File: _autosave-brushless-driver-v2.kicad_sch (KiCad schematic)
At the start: 22 parts, among them J1 Conn_01x07_Socket, J2 encoder_r, J5 encoder_l, U1 ESP32-WROOM-32E-R2

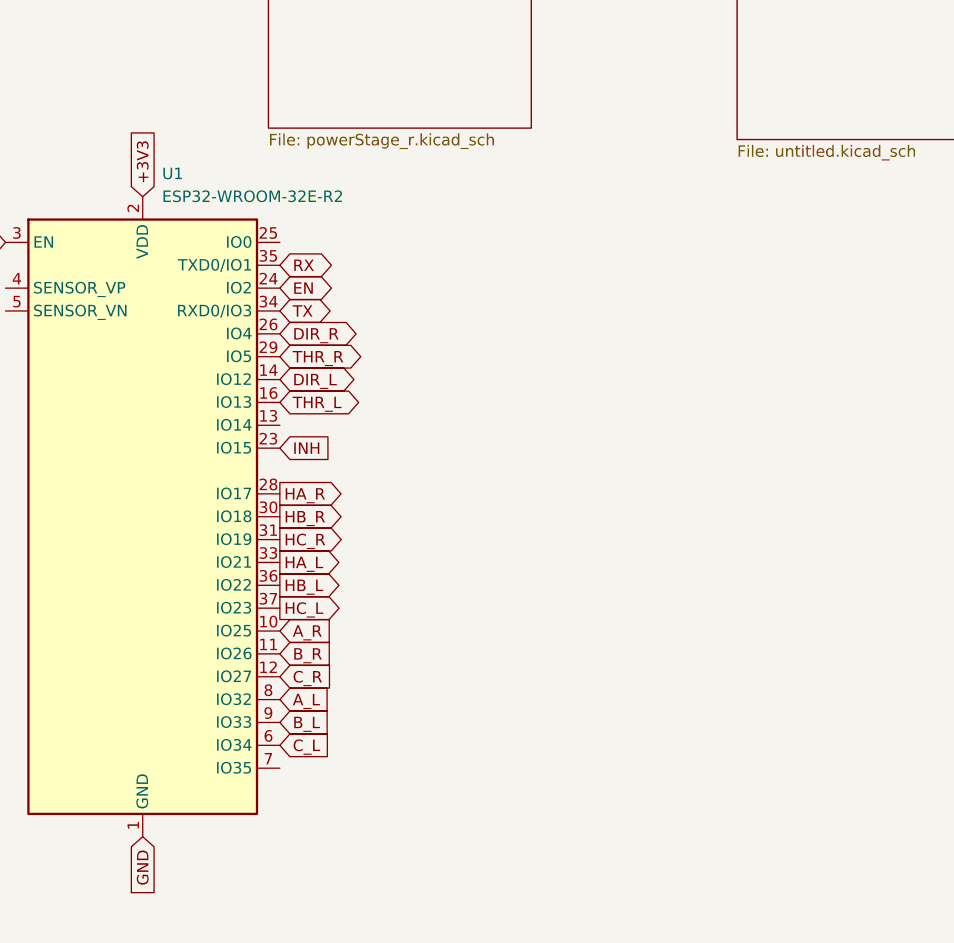
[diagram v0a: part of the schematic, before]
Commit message: controller fw added, unfinished
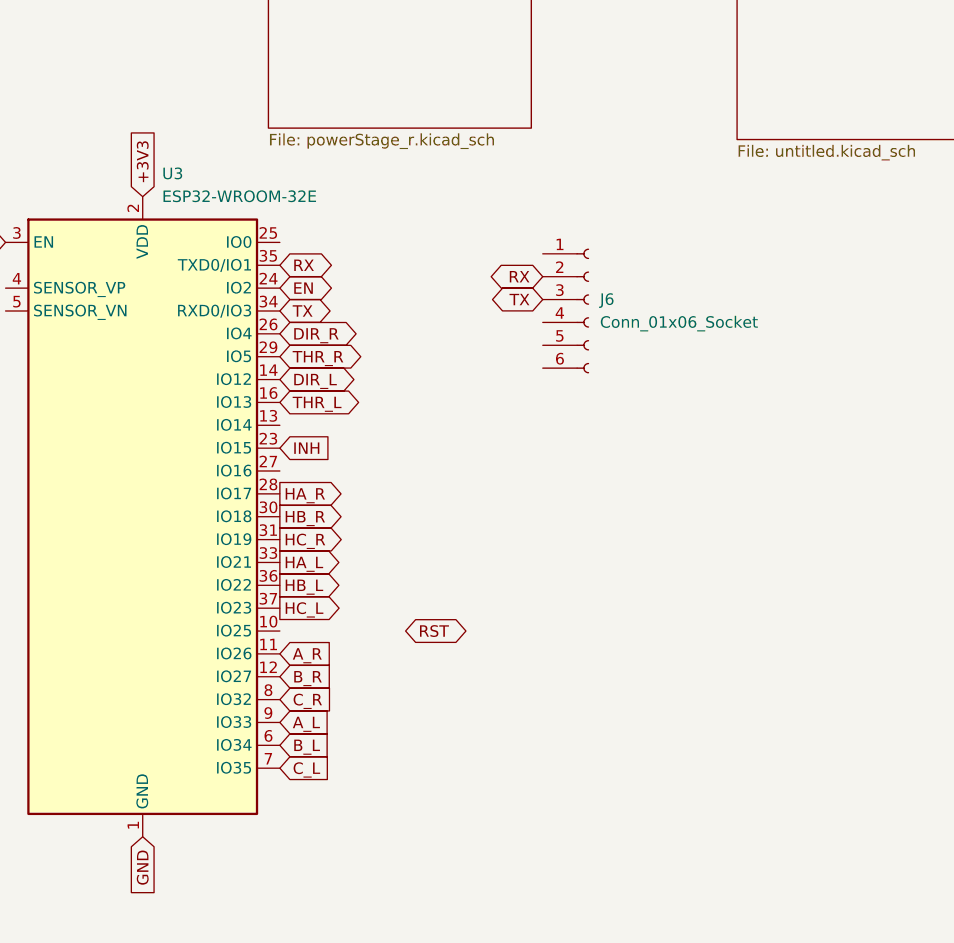
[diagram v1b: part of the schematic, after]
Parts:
- removed U1: ESP32-WROOM-32E-R2, RF_Module:ESP32-WROOM-32D, symbol RF_Module:ESP32-WROOM-32E-R2
- added J6: Conn_01x06_Socket, symbol Connector:Conn_01x06_Socket
- added U3: ESP32-WROOM-32E, RF_Module:ESP32-WROOM-32D, symbol RF_Module:ESP32-WROOM-32E
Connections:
- net +3V3: now also U3.2 (VDD), U3.3 (EN)
- net A_L: now also U3.9 (IO33)
- net A_R: now also U3.11 (IO26)
- net B_L: now also U3.6 (IO34)
- net B_R: now also U3.12 (IO27)
- net C_L: now also U3.7 (IO35)
- net C_R: now also U3.8 (IO32)
- net DIR_L: now also U3.14 (IO12)
- net DIR_R: now also U3.26 (IO4)
- net EN: now also U3.24 (IO2)
- net GND: now also U3.1 (GND), U3.15 (GND), U3.38 (GND), U3.39 (GND)
- net HA_L: now also U3.33 (IO21)
- net HA_R: now also U3.28 (IO17)
- net HB_L: now also U3.36 (IO22)
- net HB_R: now also U3.30 (IO18)
- net HC_L: now also U3.37 (IO23)
- net HC_R: now also U3.31 (IO19)
- net INH: now also U3.23 (IO15)
- net RX: now also J6.2 (Pin_2), U3.35 (TXD0/IO1)
- net THR_L: now also U3.16 (IO13)
- net THR_R: now also U3.29 (IO5)
- net TX: now also J6.3 (Pin_3), U3.34 (RXD0/IO3)
